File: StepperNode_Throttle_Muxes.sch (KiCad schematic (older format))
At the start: 6 parts

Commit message: First Revision -
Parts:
- removed P? (x2): CONN_01X08_2MNT, symbol CONN_01X08_2MNT
- added P2, P3: TE_640456-8, RLOOP_FOOTPRINTS:rLoop_TE640456-8, symbol TE_640456-8
- gave numbers to parts that had none: 4
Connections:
- net labels added: +5V_A
- net labels removed: +5VA
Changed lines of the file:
@@
 Text Label 8000 3000 0    60   ~ 0
 HE4_THROTTLE
-$Comp
-L CONN_01X08_2MNT P?
-U 1 1 5753D112
-P 11200 2400
-F 0 "P?" H 11200 2850 50  0000 C CNN
-F 1 "CONN_01X08_2MNT" V 11300 2400 50  0000 C CNN
-F 2 "" H 11200 2400 50  0000 C CNN
-F 3 "" H 11200 2400 50  0000 C CNN
-	1    11200 2400
-	1    0    0    -1
-$EndComp
 Wire Wire Line
 	11000 2050 10200 2050
@@
 Text Label 8000 6500 0    60   ~ 0
 HE8_THROTTLE
-$Comp
-L CONN_01X08_2MNT P?
-U 1 1 5753D29F
-P 11200 5900
-F 0 "P?" H 11200 6350 50  0000 C CNN
-F 1 "CONN_01X08_2MNT" V 11300 5900 50  0000 C CNN
-F 2 "" H 11200 5900 50  0000 C CNN
-F 3 "" H 11200 5900 50  0000 C CNN
-	1    11200 5900
-	1    0    0    -1
-$EndComp
 Wire Wire Line
 	11000 5550 10200 5550
@@
 STEP_DIR_CTRL
 $Comp
-L +5VA #PWR?
-U 1 1 57569503
-P 7250 1850
-F 0 "#PWR?" H 7250 1700 50  0001 C CNN
-F 1 "+5VA" H 7250 1990 50  0000 C CNN
-F 2 "" H 7250 1850 50  0000 C CNN
-F 3 "" H 7250 1850 50  0000 C CNN
-	1    7250 1850
-	1    0    0    -1
-$EndComp
-$Comp
-L +5VA #PWR?
-U 1 1 57569510
-P 7650 1150
-F 0 "#PWR?" H 7650 1000 50  0001 C CNN
-F 1 "+5VA" H 7650 1290 50  0000 C CNN
-F 2 "" H 7650 1150 50  0000 C CNN
-F 3 "" H 7650 1150 50  0000 C CNN
-	1    7650 1150
-	1    0    0    -1
-$EndComp
-$Comp
-L GNDD #PWR?
+L GNDD #PWR8
 U 1 1 57569516
 P 7050 1850
-F 0 "#PWR?" H 7050 1600 50  0001 C CNN
+F 0 "#PWR8" H 7050 1600 50  0001 C CNN
 F 1 "GNDD" H 7050 1700 50  0000 C CNN
 F 2 "" H 7050 1850 50  0000 C CNN
@@
 High = NO Channel
 $Comp
-L GNDA #PWR?
+L GNDA #PWR15
 U 1 1 5756951F
 P 7650 1450
-F 0 "#PWR?" H 7650 1200 50  0001 C CNN
+F 0 "#PWR15" H 7650 1200 50  0001 C CNN
 F 1 "GNDA" H 7650 1300 50  0000 C CNN
 F 2 "" H 7650 1450 50  0000 C CNN
@@
 $EndComp
 $Comp
-L +5VA #PWR?
-U 1 1 57569690
-P 7250 5350
-F 0 "#PWR?" H 7250 5200 50  0001 C CNN
-F 1 "+5VA" H 7250 5490 50  0000 C CNN
-F 2 "" H 7250 5350 50  0000 C CNN
-F 3 "" H 7250 5350 50  0000 C CNN
-	1    7250 5350
-	1    0    0    -1
-$EndComp
-$Comp
-L +5VA #PWR?
-U 1 1 5756969D
-P 7650 4650
-F 0 "#PWR?" H 7650 4500 50  0001 C CNN
-F 1 "+5VA" H 7650 4790 50  0000 C CNN
-F 2 "" H 7650 4650 50  0000 C CNN
-F 3 "" H 7650 4650 50  0000 C CNN
-	1    7650 4650
-	1    0    0    -1
-$EndComp
-$Comp
-L GNDD #PWR?
+L GNDD #PWR9
 U 1 1 575696A3
 P 7050 5350
-F 0 "#PWR?" H 7050 5100 50  0001 C CNN
+F 0 "#PWR9" H 7050 5100 50  0001 C CNN
 F 1 "GNDD" H 7050 5200 50  0000 C CNN
 F 2 "" H 7050 5350 50  0000 C CNN
@@
 	7150 5000 6150 5000
 $Comp
-L GNDA #PWR?
+L GNDA #PWR17
 U 1 1 575696AC
 P 7650 4950
-F 0 "#PWR?" H 7650 4700 50  0001 C CNN
+F 0 "#PWR17" H 7650 4700 50  0001 C CNN
 F 1 "GNDA" H 7650 4800 50  0000 C CNN
 F 2 "" H 7650 4950 50  0000 C CNN
@@
 STEP_DIR_CTRL
 $Comp
-L GNDA #PWR?
+L GNDA #PWR11
 U 1 1 57569B4E
 P 7200 7700
-F 0 "#PWR?" H 7200 7450 50  0001 C CNN
+F 0 "#PWR11" H 7200 7450 50  0001 C CNN
 F 1 "GNDA" H 7200 7550 50  0000 C CNN
 F 2 "" H 7200 7700 50  0000 C CNN
@@
 	7200 7700 7200 7550
 $Comp
-L GNDA #PWR?
+L GNDA #PWR10
 U 1 1 57569C1E
 P 7200 4200
-F 0 "#PWR?" H 7200 3950 50  0001 C CNN
+F 0 "#PWR10" H 7200 3950 50  0001 C CNN
 F 1 "GNDA" H 7200 4050 50  0000 C CNN
 F 2 "" H 7200 4200 50  0000 C CNN
@@
 Notes on HE throttle interface:\n1. We need to maintain electrical isolation (GND/SIG)\n2. We need to supply +12V (Fused) for the electronics to run\n3. We need RS485 comms\n4. Fwd/Rev? How? - Swap Phase A and C or set motor features to 0x01 to swap\n
 $Comp
-L MAX4948ETG+ U?
+L MAX4948ETG+ U2
 U 1 1 575A07D6
 P 6700 2050
-F 0 "U?" H 7550 2100 60  0000 C CNN
+F 0 "U2" H 7550 2100 60  0000 C CNN
 F 1 "MAX4948ETG+" H 7750 200 60  0000 C CNN
 F 2 "RLOOP_FOOTPRINTS:rLoop_QFN24_4x4mm" H 6700 1000 60  0001 C CNN
@@
 $EndComp
 $Comp
-L MAX4948ETG+ U?
+L MAX4948ETG+ U3
 U 1 1 575A08CC
 P 6700 5550
-F 0 "U?" H 7550 5600 60  0000 C CNN
+F 0 "U3" H 7550 5600 60  0000 C CNN
 F 1 "MAX4948ETG+" H 7750 3700 60  0000 C CNN
 F 2 "RLOOP_FOOTPRINTS:rLoop_QFN24_4x4mm" H 6700 4500 60  0001 C CNN
@@
 $EndComp
 $Comp
-L C_100nF_50V C?
+L C_100nF_50V C2
 U 1 1 575A2190
 P 7650 1300
-F 0 "C?" H 7675 1400 50  0000 L CNN
+F 0 "C2" H 7675 1400 50  0000 L CNN
 F 1 "C_100nF_50V" H 7675 1200 50  0000 L CNN
 F 2 "RLOOP_FOOTPRINTS:rLoop_C_0603" H 7688 1150 50  0001 C CNN
@@
 $EndComp
 $Comp
-L C_100nF_50V C?
+L C_100nF_50V C3
 U 1 1 575A22FF
 P 7650 4800
-F 0 "C?" H 7675 4900 50  0000 L CNN
+F 0 "C3" H 7675 4900 50  0000 L CNN
 F 1 "C_100nF_50V" H 7675 4700 50  0000 L CNN
 F 2 "RLOOP_FOOTPRINTS:rLoop_C_0603" H 7688 4650 50  0001 C CNN
@@
 	1    0    0    -1
 $EndComp
+$Comp
+L TE_640456-8 P2
+U 1 1 57672A7C
+P 11150 2000
+F 0 "P2" H 11200 2050 50  0000 C CNN
+F 1 "TE_640456-8" V 11300 1600 50  0000 C CNN
+F 2 "RLOOP_FOOTPRINTS:rLoop_TE640456-8" H 11200 1600 50  0001 C CNN
+F 3 "" H 11200 1600 50  0000 C CNN
+	1    11150 2000
+	1    0    0    -1
+$EndComp
+$Comp
+L TE_640456-8 P3
+U 1 1 57672BE5
+P 11150 5500
+F 0 "P3" H 11200 5550 50  0000 C CNN
+F 1 "TE_640456-8" V 11300 5100 50  0000 C CNN
+F 2 "RLOOP_FOOTPRINTS:rLoop_TE640456-8" H 11200 5100 50  0001 C CNN
+F 3 "" H 11200 5100 50  0000 C CNN
+	1    11150 5500
+	1    0    0    -1
+$EndComp
+$Comp
+L +5V_A #PWR14
+U 1 1 57672F62
+P 7650 1150
+F 0 "#PWR14" H 7650 1000 50  0001 C CNN
+F 1 "+5V_A" H 7650 1290 50  0000 C CNN
+F 2 "" H 7650 1150 60  0000 C CNN
+F 3 "" H 7650 1150 60  0000 C CNN
+	1    7650 1150
+	1    0    0    -1
+$EndComp
+$Comp
+L +5V_A #PWR12
+U 1 1 57672F82
+P 7250 1850
+F 0 "#PWR12" H 7250 1700 50  0001 C CNN
+F 1 "+5V_A" H 7250 1990 50  0000 C CNN
+F 2 "" H 7250 1850 60  0000 C CNN
+F 3 "" H 7250 1850 60  0000 C CNN
+	1    7250 1850
+	1    0    0    -1
+$EndComp
+$Comp
+L +5V_A #PWR16
+U 1 1 5767309E
+P 7650 4650
+F 0 "#PWR16" H 7650 4500 50  0001 C CNN
+F 1 "+5V_A" H 7650 4790 50  0000 C CNN
+F 2 "" H 7650 4650 60  0000 C CNN
+F 3 "" H 7650 4650 60  0000 C CNN
+	1    7650 4650
+	1    0    0    -1
+$EndComp
+$Comp
+L +5V_A #PWR13
+U 1 1 576730BE
+P 7250 5350
+F 0 "#PWR13" H 7250 5200 50  0001 C CNN
+F 1 "+5V_A" H 7250 5490 50  0000 C CNN
+F 2 "" H 7250 5350 60  0000 C CNN
+F 3 "" H 7250 5350 60  0000 C CNN
+	1    7250 5350
+	1    0    0    -1
+$EndComp

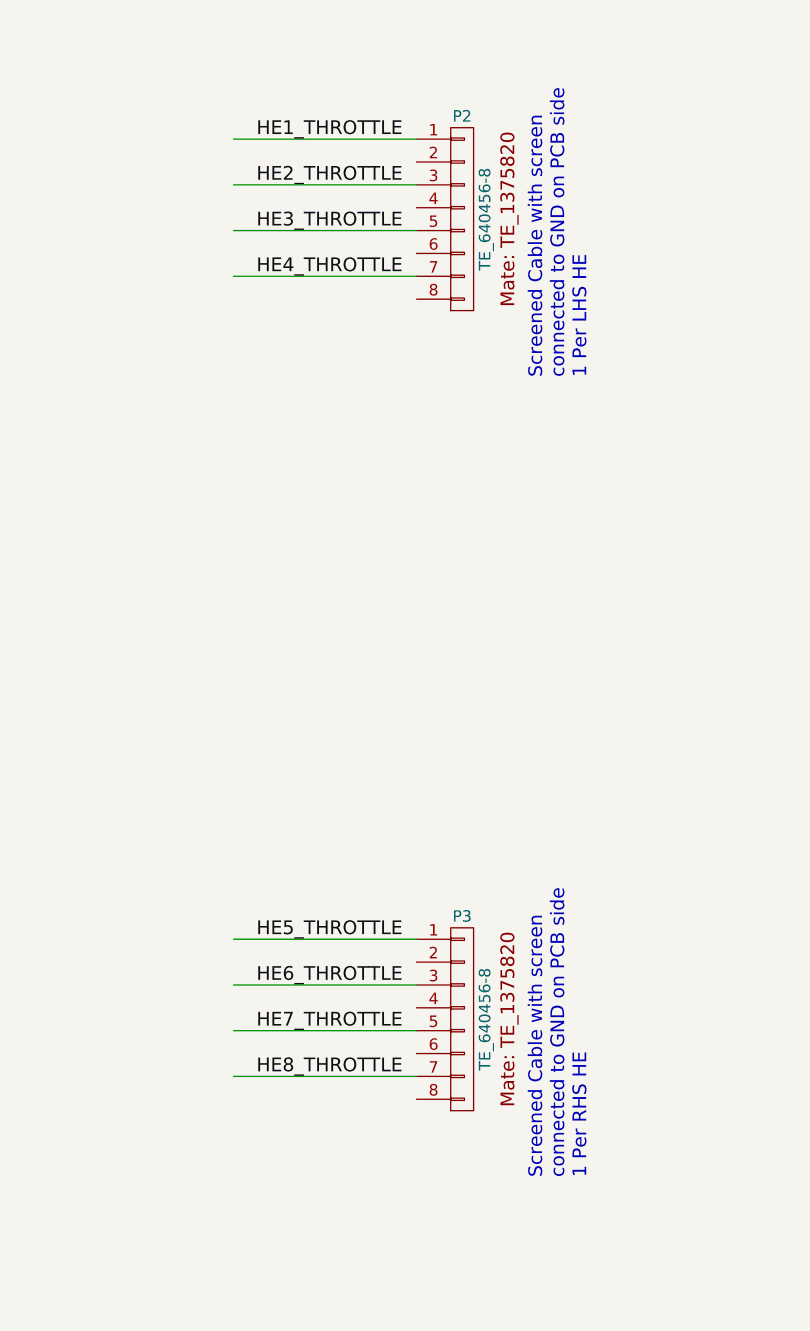
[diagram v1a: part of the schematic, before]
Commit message: Update per design review.
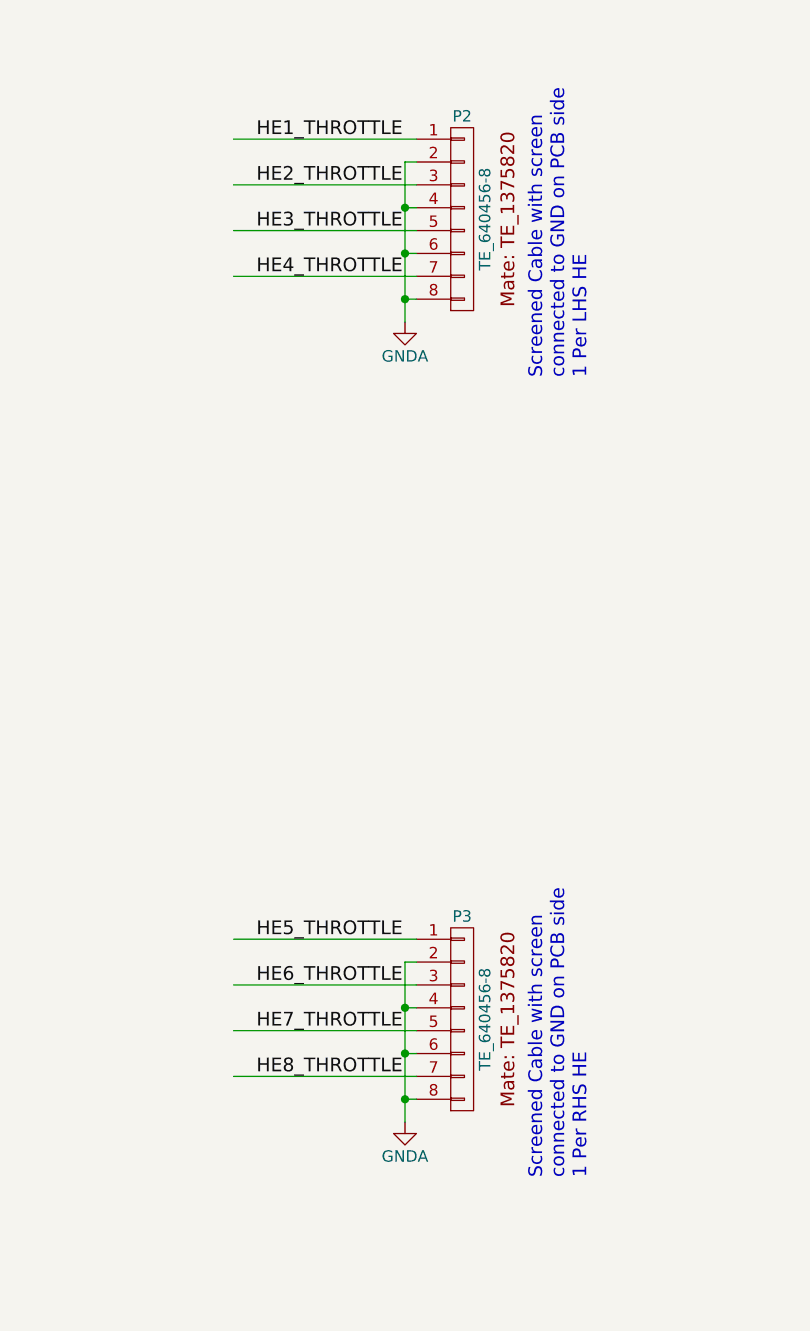
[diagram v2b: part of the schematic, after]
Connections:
- wire segments 46 -> 56
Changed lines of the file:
@@
 Title "Throttle Multiplexers"
 Date ""
-Rev "1"
+Rev "2"
 Comp ""
 Comment1 ""
@@
 	1    0    0    -1
 $EndComp
+$Comp
+L GNDA #PWR?
+U 1 1 575D0F3B
+P 10950 6350
+F 0 "#PWR?" H 10950 6100 50  0001 C CNN
+F 1 "GNDA" H 10950 6200 50  0000 C CNN
+F 2 "" H 10950 6350 50  0000 C CNN
+F 3 "" H 10950 6350 50  0000 C CNN
+	1    10950 6350
+	1    0    0    -1
+$EndComp
+Wire Wire Line
+	11000 5650 10950 5650
+Wire Wire Line
+	10950 5650 10950 6350
+Wire Wire Line
+	11000 6250 10950 6250
+Connection ~ 10950 6250
+Wire Wire Line
+	11000 6050 10950 6050
+Connection ~ 10950 6050
+Wire Wire Line
+	11000 5850 10950 5850
+Connection ~ 10950 5850
+$Comp
+L GNDA #PWR?
+U 1 1 575D10B7
+P 10950 2850
+F 0 "#PWR?" H 10950 2600 50  0001 C CNN
+F 1 "GNDA" H 10950 2700 50  0000 C CNN
+F 2 "" H 10950 2850 50  0000 C CNN
+F 3 "" H 10950 2850 50  0000 C CNN
+	1    10950 2850
+	1    0    0    -1
+$EndComp
+Wire Wire Line
+	10950 2150 10950 2850
+Wire Wire Line
+	11000 2150 10950 2150
+Wire Wire Line
+	11000 2350 10950 2350
+Connection ~ 10950 2350
+Wire Wire Line
+	11000 2550 10950 2550
+Connection ~ 10950 2550
+Wire Wire Line
+	11000 2750 10950 2750
+Connection ~ 10950 2750
 $EndSCHEMATC
